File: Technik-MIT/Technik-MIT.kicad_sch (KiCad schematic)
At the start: 26 parts, among them J1 USB_C_Receptacle_USB2.0, U1 RP2040, U2 TVS0500DRV, U3 NCP1117-3.3_SOT223, U4 USBLC6-2SC6, U5 W25Q32JVSS, Y1 Crystal

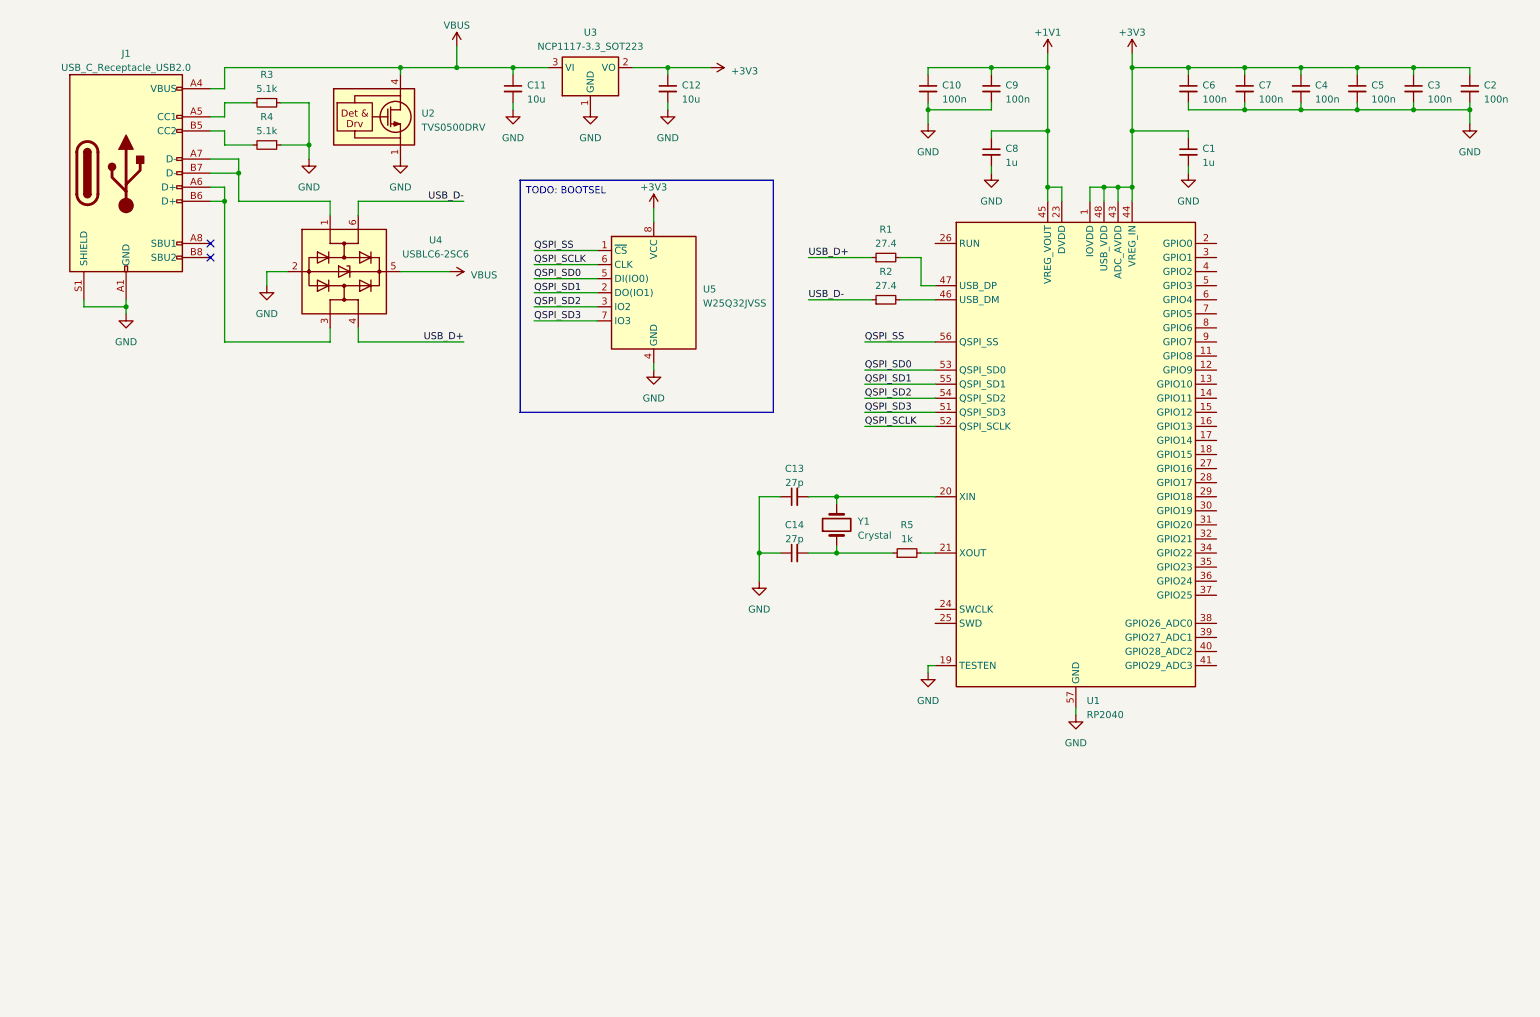
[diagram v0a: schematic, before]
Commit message: Update PCB schematic
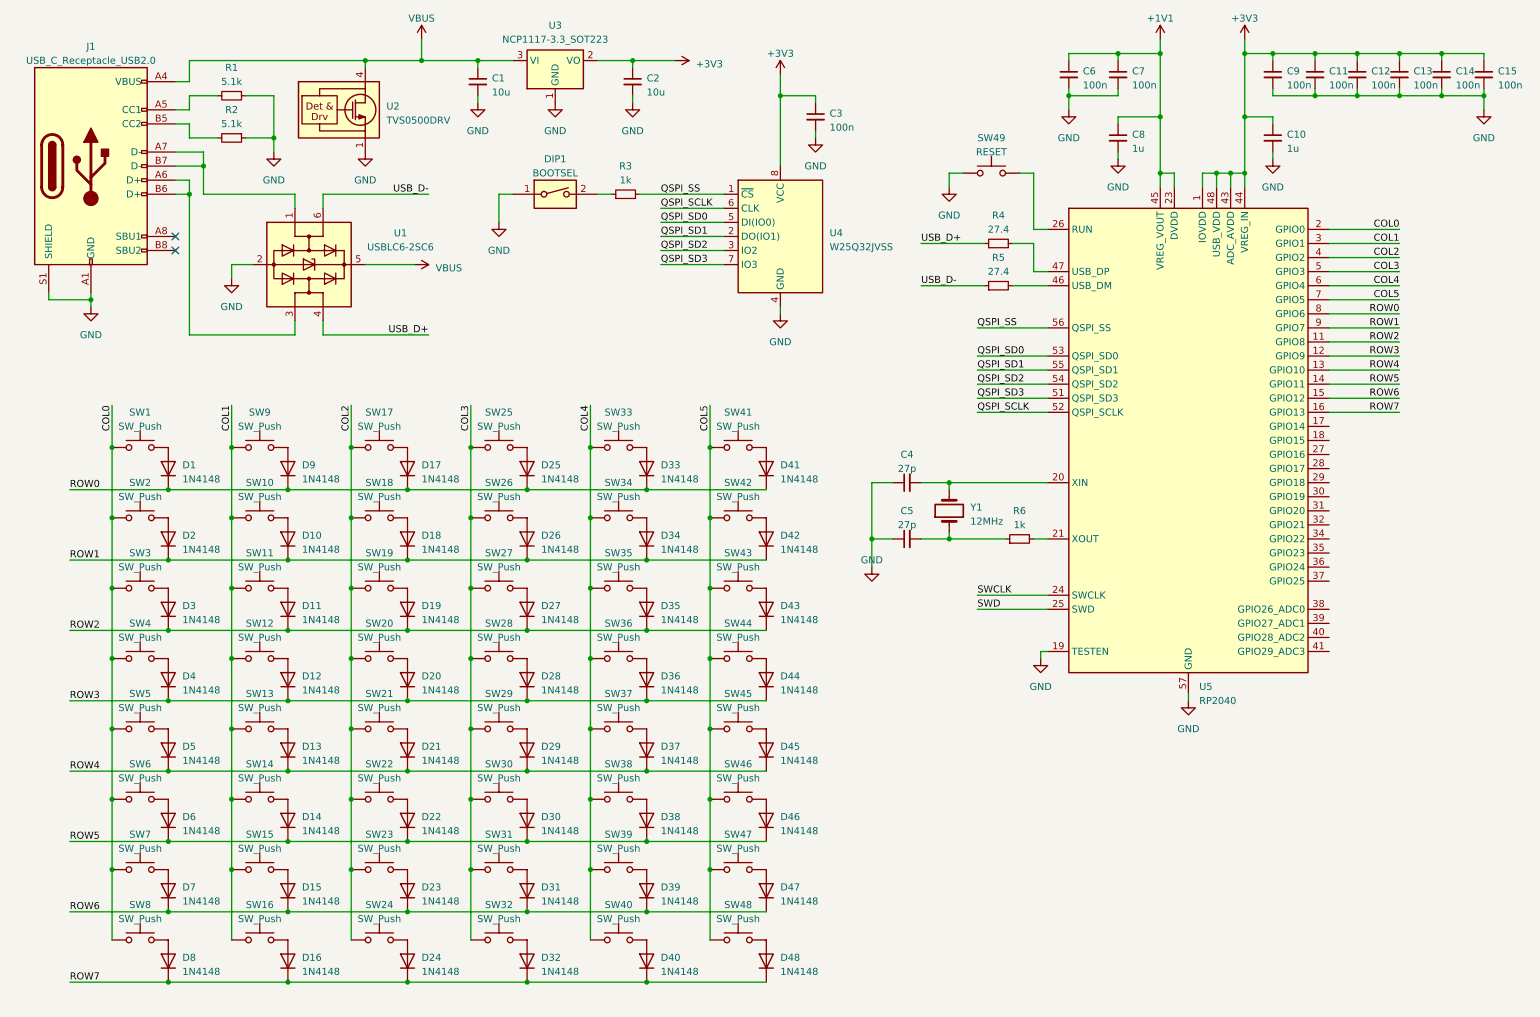
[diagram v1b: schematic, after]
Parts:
- added C3: 100n, symbol Device:C_Small
- added D1, D10, D11, D12, D13, D14, D15, D16, D17, D18, D19, D2, D20, D21, D22, D23, D24, D25, D26, D27, D28, D29, D3, D30, D31, D32, D33, D34, D35, D36, D37, D38, D39, D4, D40, D41, D42, D43, D44, D45, D46, D47, D48, D5, D6, D7, D8, D9: 1N4148, Diode_THT:D_DO-35_SOD27_P7.62mm_Horizontal, symbol Diode:1N4148
- added DIP1: BOOTSEL, symbol Switch:SW_DIP_x01
- added R3: 1k, symbol Device:R_Small
- added SW1, SW10, SW11, SW12, SW13, SW14, SW15, SW16, SW17, SW18, SW19, SW2, SW20, SW21, SW22, SW23, SW24, SW25, SW26, SW27, SW28, SW29, SW3, SW30, SW31, SW32, SW33, SW34, SW35, SW36, SW37, SW38, SW39, SW4, SW40, SW41, SW42, SW43, SW44, SW45, SW46, SW47, SW48, SW5, SW6, SW7, SW8, SW9: SW_Push, symbol Switch:SW_Push
- added SW49: RESET, symbol Switch:SW_Push
- Y1: value Crystal -> 12MHz
- renumbered C11 to C1, C1 to C10, C7 to C11, C4 to C12, C5 to C13, C3 to C14, C2 to C15, C12 to C2, C13 to C4, C14 to C5, C10 to C6, C9 to C7, C6 to C9, R3 to R1, R4 to R2, R1 to R4, R2 to R5, R5 to R6, U4 to U1, U5 to U4, U1 to U5
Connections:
- net +3V3: now also C3.1
- net GND: now also C3.2, DIP1.1, SW49.1
- net QSPI_SS: now also R3.2
- net ROW2: now reaches U5.11 (GPIO8)
- net ROW2: now also D11.1 (K), D19.1 (K), D27.1 (K), D3.1 (K), D35.1 (K), D43.1 (K)
- net ROW3: now reaches U5.12 (GPIO9)
- net ROW3: now also D12.1 (K), D20.1 (K), D28.1 (K), D36.1 (K), D4.1 (K), D44.1 (K)
- net ROW4: now reaches U5.13 (GPIO10)
- net ROW4: now also D13.1 (K), D21.1 (K), D29.1 (K), D37.1 (K), D45.1 (K), D5.1 (K)
- net ROW5: now reaches U5.14 (GPIO11)
- net ROW5: now also D14.1 (K), D22.1 (K), D30.1 (K), D38.1 (K), D46.1 (K), D6.1 (K)
- net ROW6: now reaches U5.15 (GPIO12)
- net ROW6: now also D15.1 (K), D23.1 (K), D31.1 (K), D39.1 (K), D47.1 (K), D7.1 (K)
- net ROW7: now reaches U5.16 (GPIO13)
- net ROW7: now also D16.1 (K), D24.1 (K), D32.1 (K), D40.1 (K), D48.1 (K), D8.1 (K)
- net COL0: now reaches U5.2 (GPIO0)
- net COL0: now also SW1.1, SW2.1, SW3.1, SW4.1, SW5.1, SW6.1, SW7.1, SW8.1
- net SWCLK: now reaches U5.24 (SWCLK)
- net SWD: now reaches U5.25 (SWD)
- net at U5.26 (RUN): now also SW49.2
- net COL1: now reaches U5.3 (GPIO1)
- net COL1: now also SW10.1, SW11.1, SW12.1, SW13.1, SW14.1, SW15.1, SW16.1, SW9.1
- net COL2: now reaches U5.4 (GPIO2)
- net COL2: now also SW17.1, SW18.1, SW19.1, SW20.1, SW21.1, SW22.1, SW23.1, SW24.1
- net COL3: now reaches U5.5 (GPIO3)
- net COL3: now also SW25.1, SW26.1, SW27.1, SW28.1, SW29.1, SW30.1, SW31.1, SW32.1
- net COL4: now reaches U5.6 (GPIO4)
- net COL4: now also SW33.1, SW34.1, SW35.1, SW36.1, SW37.1, SW38.1, SW39.1, SW40.1
- net COL5: now reaches U5.7 (GPIO5)
- net COL5: now also SW41.1, SW42.1, SW43.1, SW44.1, SW45.1, SW46.1, SW47.1, SW48.1
- net ROW0: now reaches U5.8 (GPIO6)
- net ROW0: now also D1.1 (K), D17.1 (K), D25.1 (K), D33.1 (K), D41.1 (K), D9.1 (K)
- net ROW1: now reaches U5.9 (GPIO7)
- net ROW1: now also D10.1 (K), D18.1 (K), D2.1 (K), D26.1 (K), D34.1 (K), D42.1 (K)
- new net: D15.2 (A), SW15.2
- new net: D33.2 (A), SW33.2
- new net: D16.2 (A), SW16.2
- new net: D14.2 (A), SW14.2
- new net: D30.2 (A), SW30.2
- new net: D11.2 (A), SW11.2
- new net: D23.2 (A), SW23.2
- new net: D1.2 (A), SW1.2
- new net: D45.2 (A), SW45.2
- new net: D32.2 (A), SW32.2
- new net: D41.2 (A), SW41.2
- new net: D48.2 (A), SW48.2
- new net: D22.2 (A), SW22.2
- new net: D29.2 (A), SW29.2
- new net: D21.2 (A), SW21.2
- new net: D17.2 (A), SW17.2
- new net: D12.2 (A), SW12.2
- new net: D8.2 (A), SW8.2
- new net: D25.2 (A), SW25.2
- new net: D18.2 (A), SW18.2
- new net: DIP1.2, R3.1
- new net: D36.2 (A), SW36.2
- new net: D24.2 (A), SW24.2
- new net: D9.2 (A), SW9.2
- new net: D2.2 (A), SW2.2
- new net: D38.2 (A), SW38.2
- new net: D35.2 (A), SW35.2
- new net: D43.2 (A), SW43.2
- new net: D19.2 (A), SW19.2
- new net: D31.2 (A), SW31.2
- new net: D10.2 (A), SW10.2
- new net: D13.2 (A), SW13.2
- new net: D39.2 (A), SW39.2
- new net: D27.2 (A), SW27.2
- new net: D26.2 (A), SW26.2
- new net: D47.2 (A), SW47.2
- new net: D28.2 (A), SW28.2
- new net: D40.2 (A), SW40.2
- new net: D37.2 (A), SW37.2
- new net: D4.2 (A), SW4.2
- new net: D46.2 (A), SW46.2
- new net: D6.2 (A), SW6.2
- new net: D3.2 (A), SW3.2
- new net: D42.2 (A), SW42.2
- new net: D34.2 (A), SW34.2
- new net: D7.2 (A), SW7.2
- new net: D20.2 (A), SW20.2
- new net: D44.2 (A), SW44.2
- new net: D5.2 (A), SW5.2
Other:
- moved on the sheet: C1, C10, C11, C12, C13, C14, C15, C2, C4, C5, C6, C7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

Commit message: Update PCB
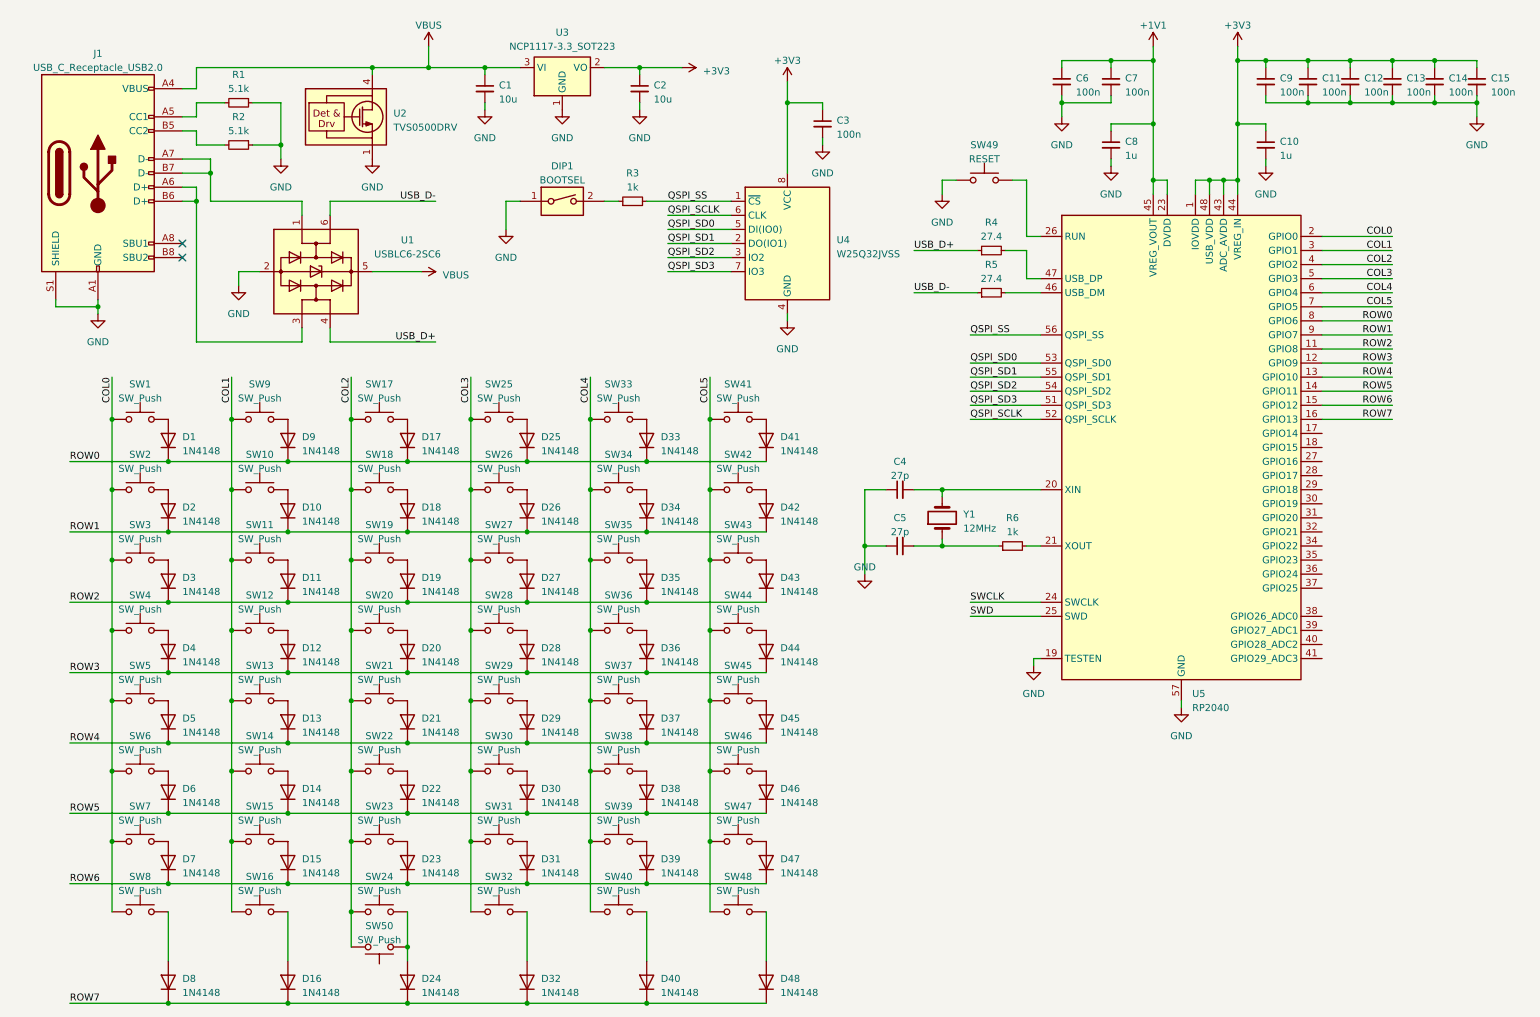
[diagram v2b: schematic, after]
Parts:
- added SW50: SW_Push, kbd:ChocV1_Hotswap, symbol Switch:SW_Push
- C1, C10, C11, C12, C13, C14, C15, C2, C3, C4, C5, C6, C7, C8, C9: footprint (none) -> Capacitor_SMD:C_0402_1005Metric
- D1, D10, D11, D12, D13, D14, D15, D16, D17, D18, D19, D2, D20, D21, D22, D23, D24, D25, D26, D27, D28, D29, D3, D30, D31, D32, D33, D34, D35, D36, D37, D38, D39, D4, D40, D41, D42, D43, D44, D45, D46, D47, D48, D5, D6, D7, D8, D9: footprint Diode_THT:D_DO-35_SOD27_P7.62mm_Horizontal -> Diode_SMD:D_SOD-123
- DIP1: footprint (none) -> Button_Switch_SMD:SW_DIP_SPSTx01_Slide_6.7x4.1mm_W8.61mm_P2.54mm_LowProfile
- J1: footprint (none) -> Connector_USB:USB_C_Receptacle_Molex_105450-0101
- R1, R2, R3, R4, R5, R6: footprint (none) -> Resistor_SMD:R_0402_1005Metric
- SW1, SW10, SW11, SW12, SW13, SW14, SW15, SW16, SW17, SW18, SW19, SW2, SW20, SW21, SW22, SW23, SW24, SW25, SW26, SW27, SW28, SW29, SW3, SW30, SW31, SW32, SW33, SW34, SW35, SW36, SW37, SW38, SW39, SW4, SW40, SW41, SW42, SW43, SW44, SW45, SW46, SW47, SW48, SW5, SW6, SW7, SW8, SW9: footprint (none) -> kbd:ChocV1_Hotswap
- SW49: footprint (none) -> Button_Switch_SMD:SW_SPST_B3U-1000P
- Y1: footprint (none) -> Crystal:Crystal_SMD_7050-4Pin_7.0x5.0mm
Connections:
- net COL2: now also SW50.2
- net at D24.2 (A), SW24.2: now also SW50.1
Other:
- moved on the sheet: C1, C10, C11, C12, C13, C14, C15, C2, C3, C4, C5, C6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
